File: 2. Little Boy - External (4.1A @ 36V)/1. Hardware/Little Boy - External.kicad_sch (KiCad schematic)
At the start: 83 parts, among them J1 TESTPOINT, J10 MOT_B, J11 MOT_A, J12 TESTPOINT, J13 Control_In, J14 Control_In, J15 Conn_01x06_MountingPin, J16 Conn_01x06_MountingPin, J17 TESTPOINT, J2 TESTPOINT, J3 TESTPOINT, J4 Prog_IN, J5 Conn_01x06_MountingPin, J6 TESTPOINT, J7 TESTPOINT, J8 Power_In, J9 Power_In, U1 STM32G0B1CBTx, U2 LMR33630CDDA, U3 TJA1051T-3, U4 TLV76733DRVx, U5 MA730, U6 W25Q128JVS, U7 DRV8251DDAR, U8 AS5600-ASOT, Y1 25 MHz

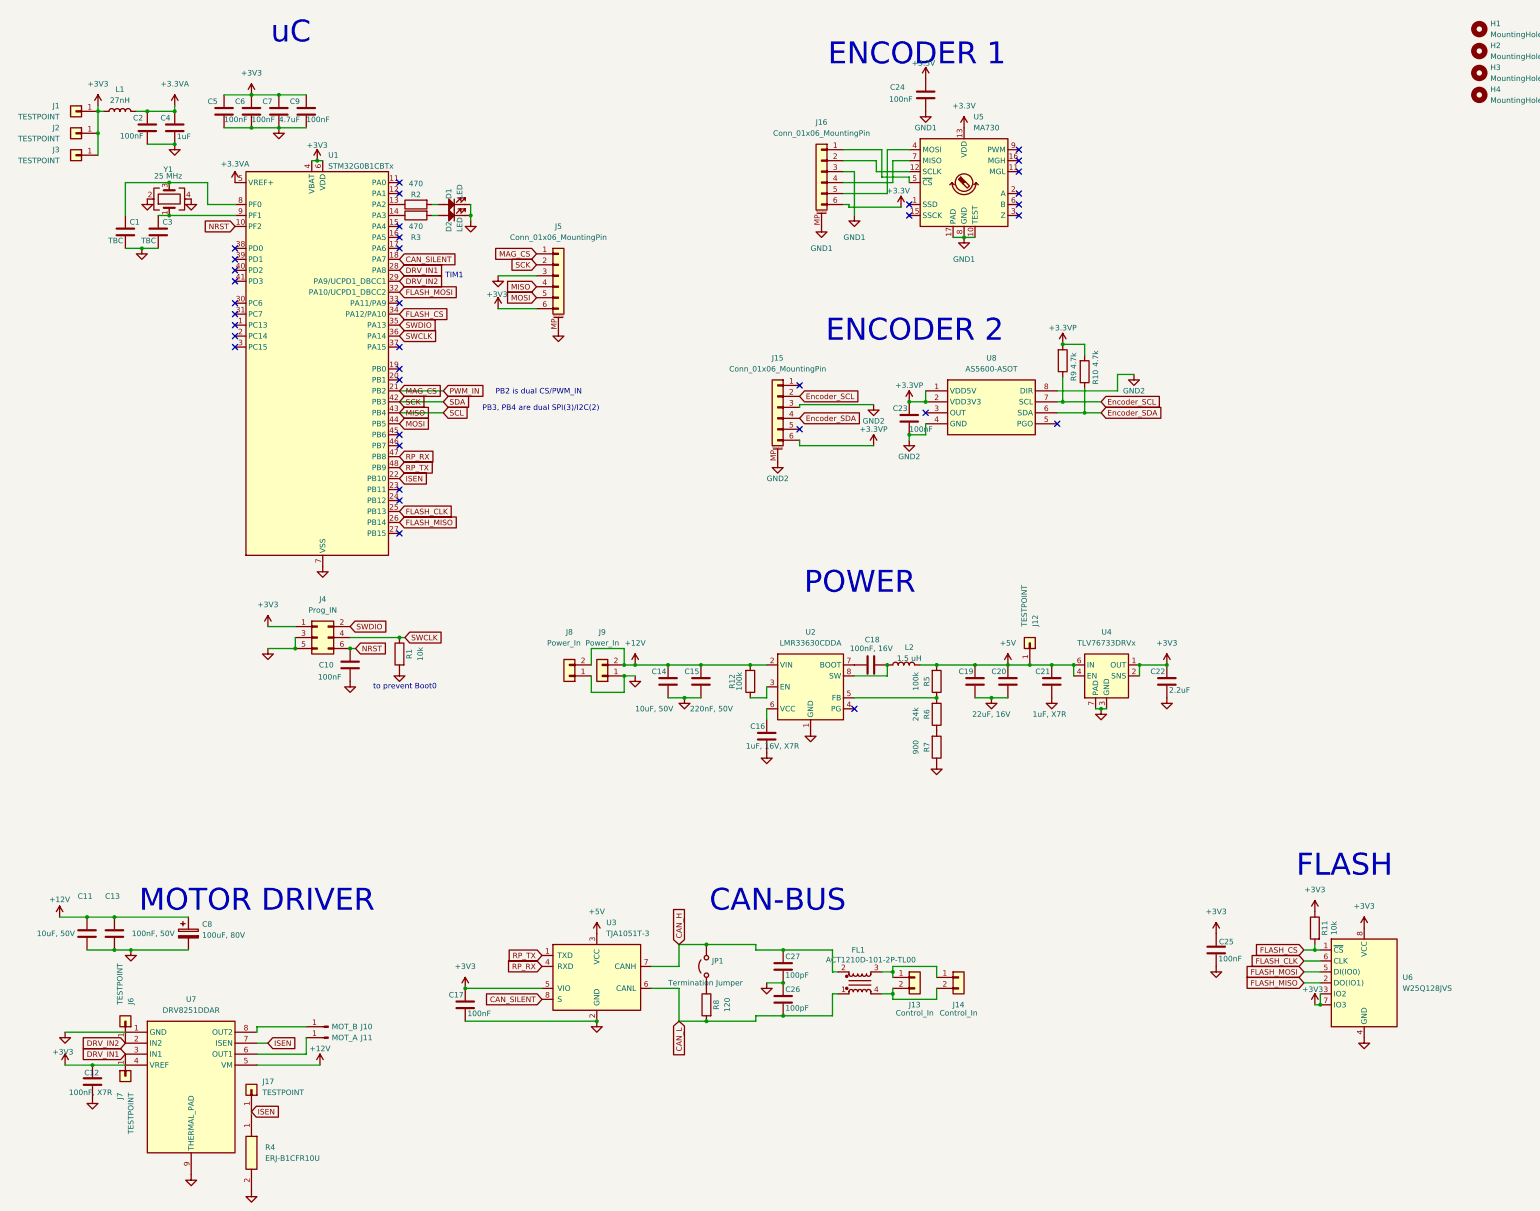
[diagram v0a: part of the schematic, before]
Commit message: big update
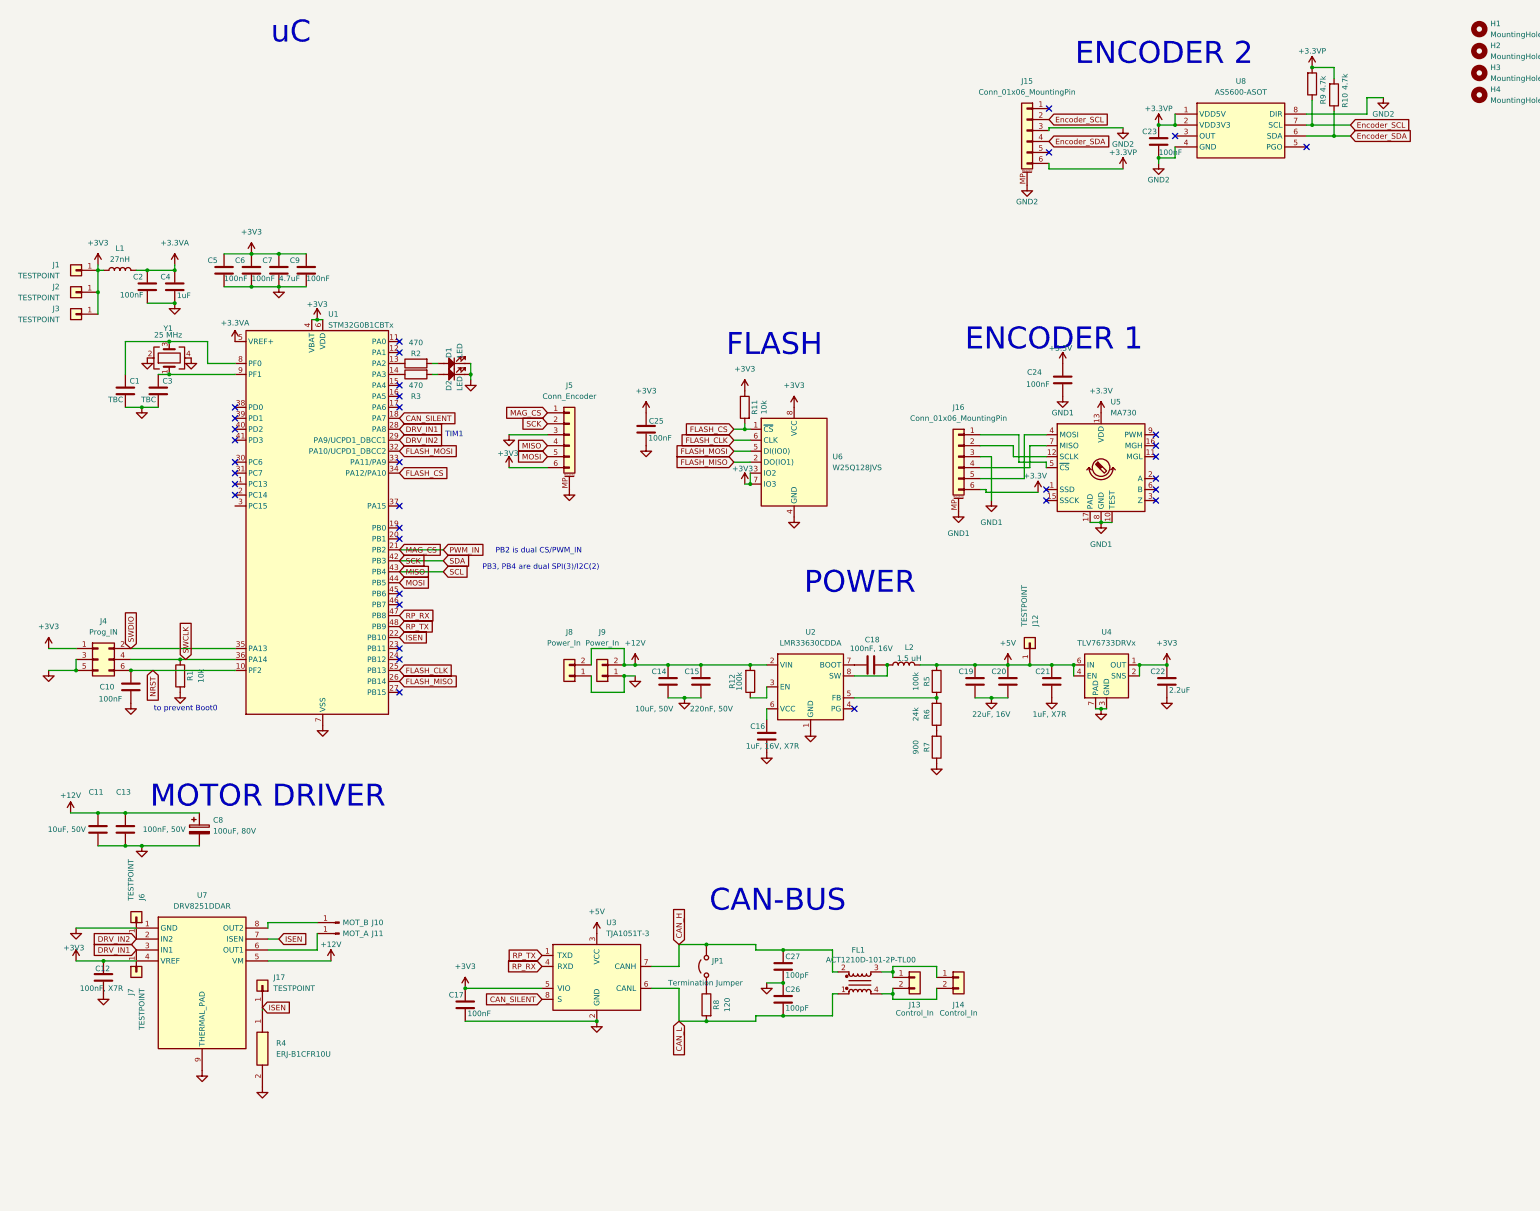
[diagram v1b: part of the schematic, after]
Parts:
- J5: value Conn_01x06_MountingPin -> Conn_Encoder
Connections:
- no-connect marks 36 -> 35
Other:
- moved on the sheet: C1, C10, C11, C12, C13, C2, C23, C24, C25, C3, C4, C5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
